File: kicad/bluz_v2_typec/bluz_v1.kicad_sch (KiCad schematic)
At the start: 76 parts, among them J10 Conn, J11 Conn, J12 BTAnt, J2 Conn, J3 Conn, J4 Conn, J5 Conn, J6 Conn, J7 Conn, J8 Conn, J9 USB_C_Receptacle_PowerOnly_6P, M1 Z3OC1T8219731, Q2 RUM002N05, SW1 SW_DPDT_x2, U1 MCP73831, U3 TLV3201AIDCK, U4 AP3015KTR, U5 MCP1700-1.8, U6 PAM8904EGPR, U7 TPS627451DSSR, Y1 NX1612SA-32MHz, Y2 NX2012SA-32.768

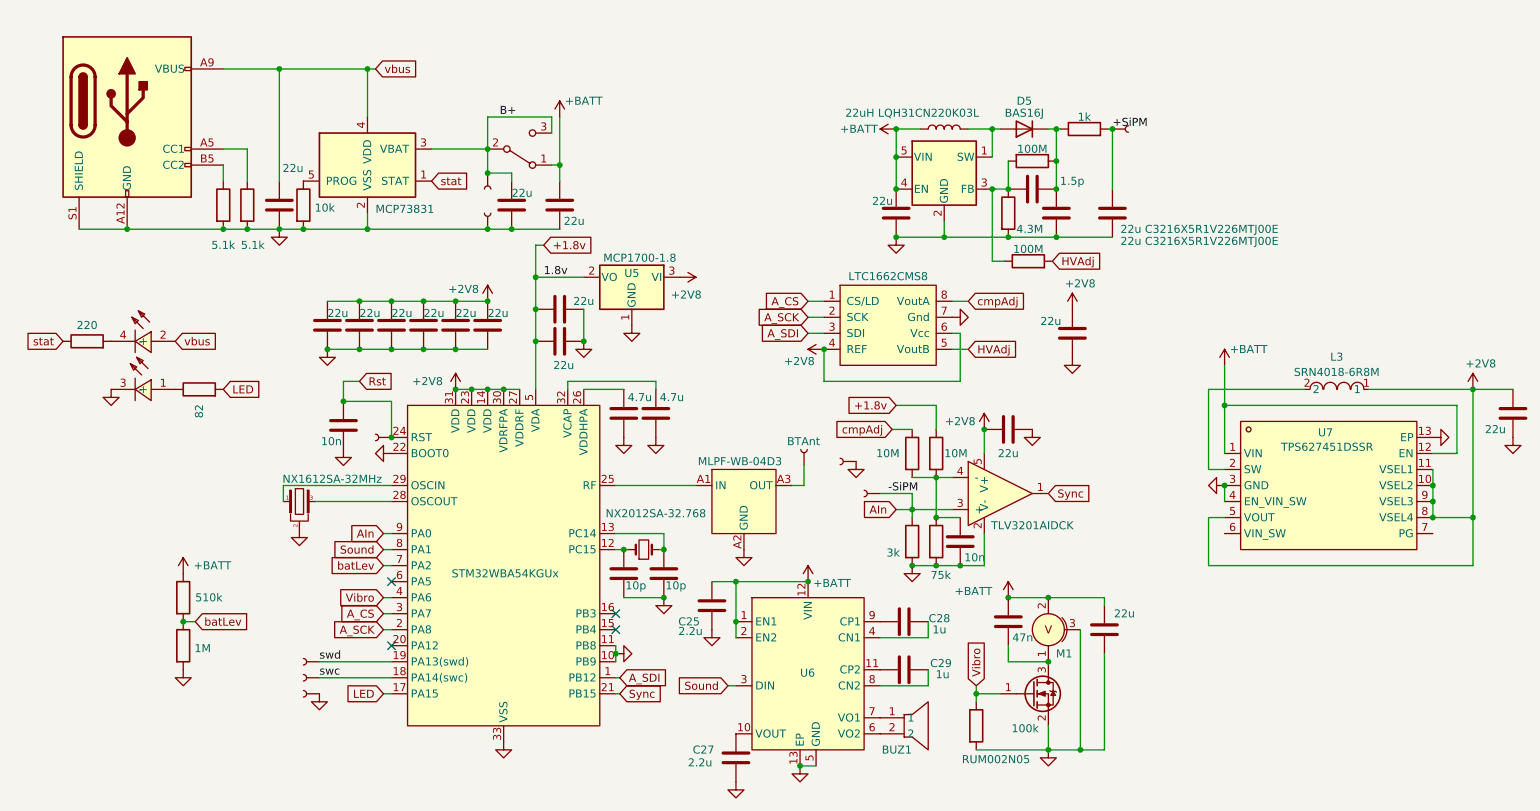
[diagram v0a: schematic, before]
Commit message: изменено:      kicad/bluz_v2_typec/bluz_v1.kicad_prl 	изменено:      kicad/bluz_v2_typec/bluz_v1.kicad_sch
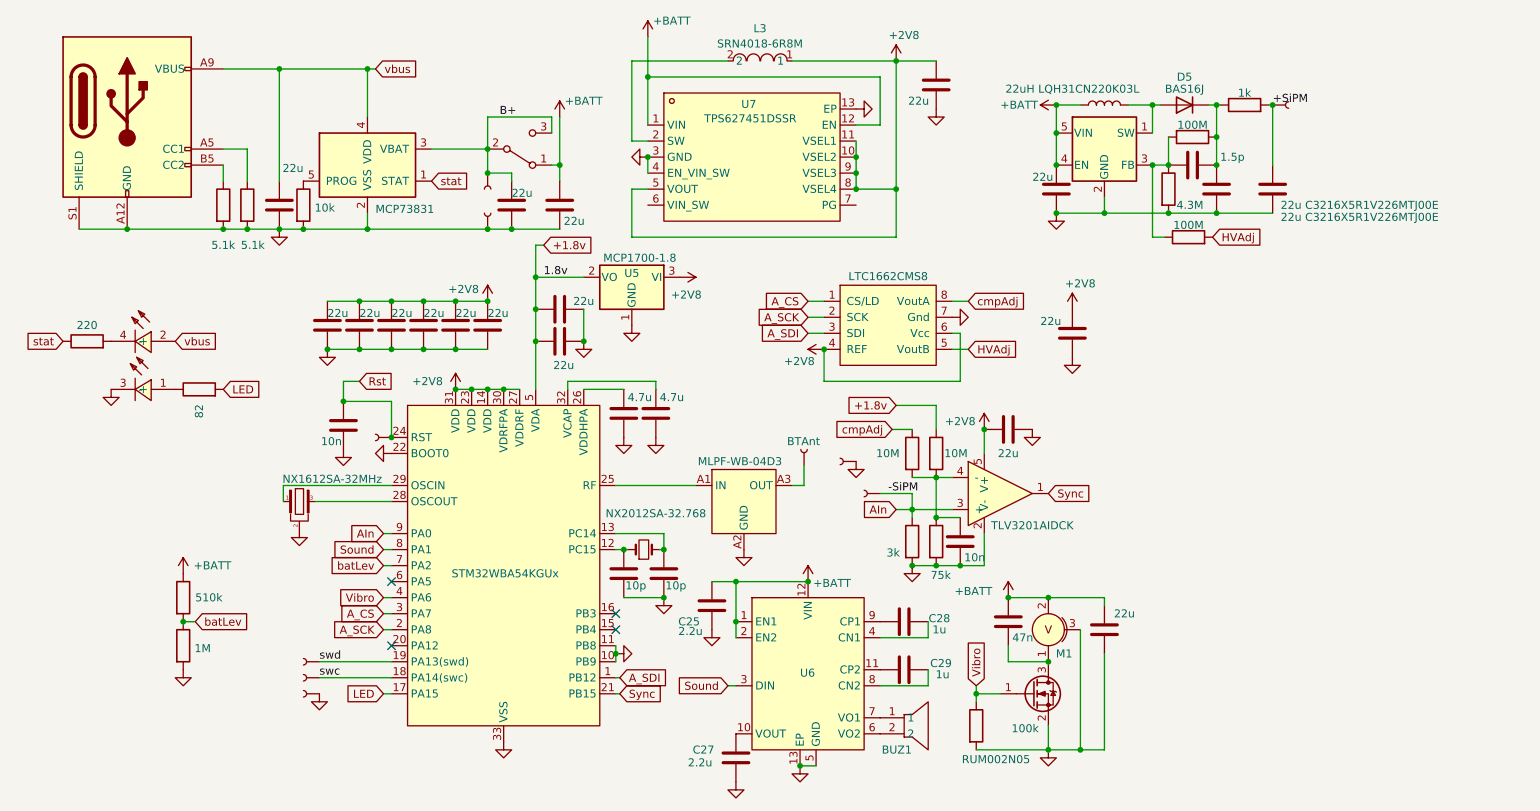
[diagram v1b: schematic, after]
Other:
- moved on the sheet: D5, L3, U7
